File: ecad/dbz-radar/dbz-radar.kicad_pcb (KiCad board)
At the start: 4 copper layers, 125.2 x 122.2 mm, 139 parts, among them J1 B2B-PH-SM4-TB, J2 USB4220-03-0880-C, J3 XF2M-4015-1A, J4 533980271, J5 DNI, Q1 Q_PMOS, SW1 SKRPACE010, SW2 SKRPACE010, SW3 1-825027-7, U1 USBLC6-2SC6, U2 TPS61169, U3 MCP738311/2, U4 MAX17048/9, U5 AP2112K-3.3, U6 PCA9554, U7 MAX98357A, U8 ESP32-S3-WROOM-1-N16R8

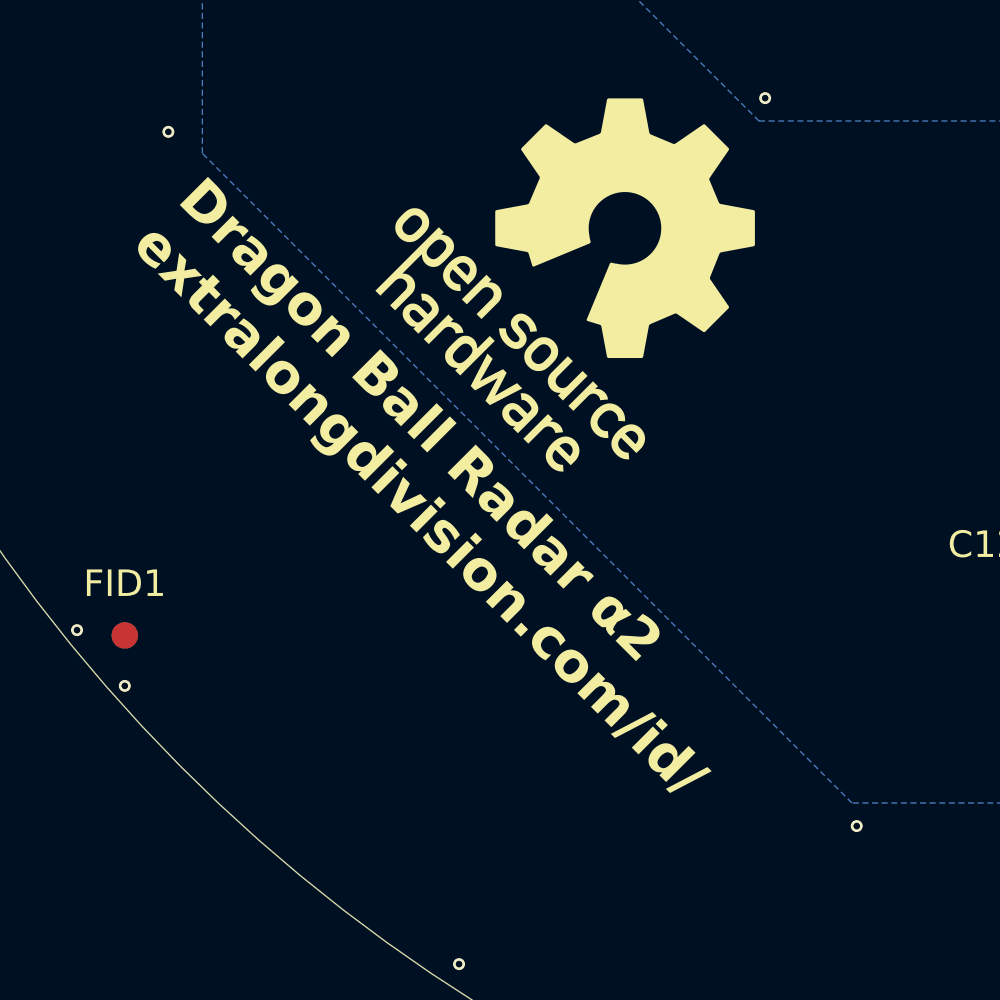
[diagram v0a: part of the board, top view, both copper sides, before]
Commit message: make production files for V1.2
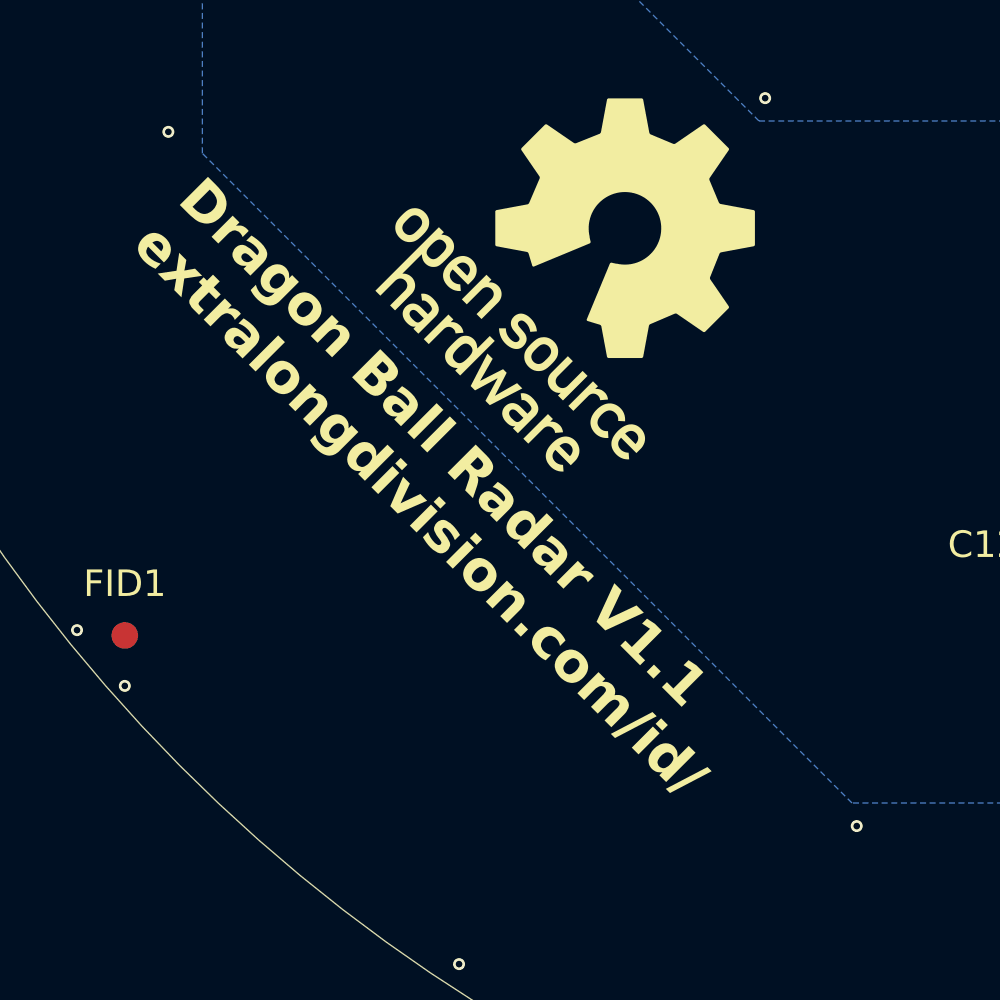
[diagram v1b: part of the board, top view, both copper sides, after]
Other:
- board text added: "Dragon Ball Radar V1.1 extralongdivision.com/id/"
- board text removed: "Dragon Ball Radar α2 extralongdivision.com/id/"
